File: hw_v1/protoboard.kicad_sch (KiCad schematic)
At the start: 17 parts, among them J15 Conn_01x03, J2 Conn_01x05, J3 Conn_01x05, J4 Conn_01x05, J5 Conn_01x03, J6 Conn_01x04

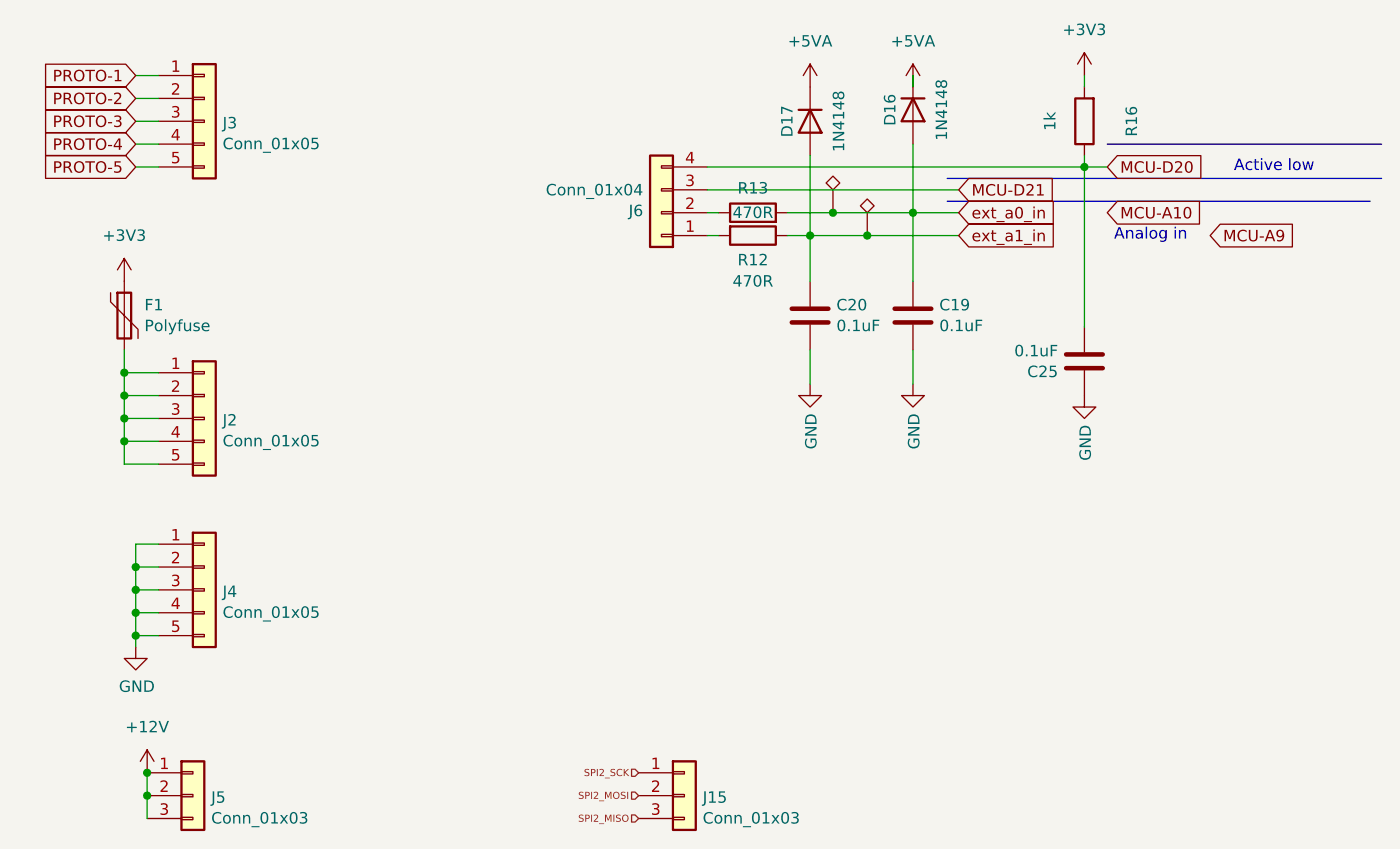
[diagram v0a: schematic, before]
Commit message: finish pcb layout
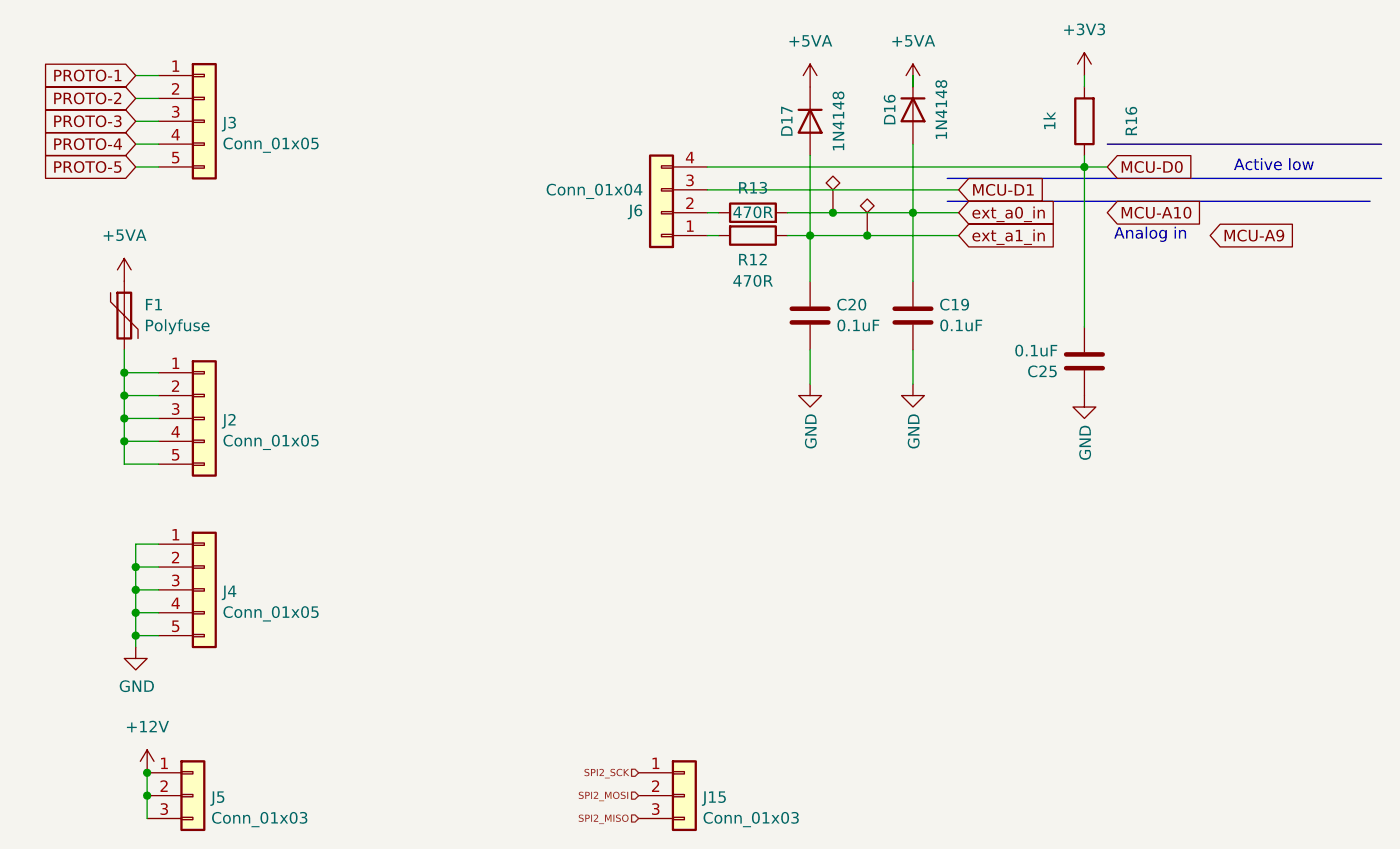
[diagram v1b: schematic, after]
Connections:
- net +3V3: no longer F1.1
- net +5VA: now also F1.1
- net MCU-D20 renamed MCU-D0
- net MCU-D21 renamed MCU-D1
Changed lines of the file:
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@@
 		)
 	)
-	(global_label "MCU-D20"
+	(global_label "MCU-D0"
 		(shape input)
 		(at 170.18 52.07 0)
@@
 		)
 	)
-	(global_label "MCU-D21"
+	(global_label "MCU-D1"
 		(shape input)
 		(at 153.67 54.61 0)
@@
 	(symbol
 		(lib_id "power:+3V3")
-		(at 60.96 64.77 0)
-		(unit 1)
-		(exclude_from_sim no)
-		(in_bom yes)
-		(on_board yes)
-		(dnp no)
-		(fields_autoplaced yes)
-		(property "Reference" "#PWR045"
-			(at 60.96 68.58 0)
-			(effects
-				(font
-					(size 1.27 1.27)
-				)
-				(hide yes)
-			)
-		)
-		(property "Value" "+3V3"
-			(at 60.96 59.69 0)
-			(effects
-				(font
-					(size 1.27 1.27)
-				)
-			)
-		)
-		(property "Footprint" ""
-			(at 60.96 64.77 0)
-			(effects
-				(font
-					(size 1.27 1.27)
-				)
-				(hide yes)
-			)
-		)
-		(property "Datasheet" ""
-			(at 60.96 64.77 0)
-			(effects
-				(font
-					(size 1.27 1.27)
-				)
-				(hide yes)
-			)
-		)
-		(property "Description" "Power symbol creates a global label with name \"+3V3\""
-			(at 60.96 64.77 0)
-			(effects
-				(font
-					(size 1.27 1.27)
-				)
-				(hide yes)
-			)
-		)
-		(pin "1"
-		)
-		(instances
-			(project "hw_v1"
-				(path "/b3feb07e-be80-40e1-bd13-6cd54c2f8b0c/019e8a83-2b05-42df-8207-97dcaa5a8956"
-					(reference "#PWR045")
-					(unit 1)
-				)
-			)
-		)
-	)
-	(symbol
-		(lib_id "power:+3V3")
 		(at 167.64 41.91 0)
 		(unit 1)
@@
 					(unit 1)
 				)
+			)
+		)
+	)
+	(symbol
+		(lib_id "power:+5VA")
+		(at 60.96 64.77 0)
+		(unit 1)
+		(exclude_from_sim no)
+		(in_bom yes)
+		(on_board yes)
+		(dnp no)
+		(fields_autoplaced yes)
+		(property "Reference" "#PWR0153"
+			(at 60.96 68.58 0)
+			(effects
+				(font
+					(size 1.27 1.27)
+				)
+				(hide yes)
+			)
+		)
+		(property "Value" "+5VA"
+			(at 60.96 59.69 0)
+			(effects
+				(font
+					(size 1.27 1.27)
+				)
+			)
+		)
+		(property "Footprint" ""
+			(at 60.96 64.77 0)
+			(effects
+				(font
+					(size 1.27 1.27)
+				)
+				(hide yes)
+			)
+		)
+		(property "Datasheet" ""
+			(at 60.96 64.77 0)
+			(effects
+				(font
+					(size 1.27 1.27)
+				)
+				(hide yes)
+			)
+		)
+		(property "Description" "Power symbol creates a global label with name \"+5VA\""
+			(at 60.96 64.77 0)
+			(effects
+				(font
+					(size 1.27 1.27)
+				)
+				(hide yes)
+			)
+		)
+		(pin "1"
+		)
+		(instances
+			(project "hw_v1"
+				(path "/b3feb07e-be80-40e1-bd13-6cd54c2f8b0c/019e8a83-2b05-42df-8207-97dcaa5a8956"
+					(reference "#PWR0153")
+					(unit 1)
+				)
